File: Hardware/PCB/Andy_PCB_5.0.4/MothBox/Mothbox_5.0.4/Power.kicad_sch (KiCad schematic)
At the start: 50 parts, among them J1 DB141V-2.54-4P, J2 DB141V-2.54-4P, J3 DB141V-2.54-4P, Q1 AP30P30Q, Q10 AP30P30Q, Q2 AO3400A, Q8 AP30P30Q, SW2 KH-6X6X5H-STM, U1 Place Holder voltage regulator, U2 XL4015E1, U3 INA219BIDCNT

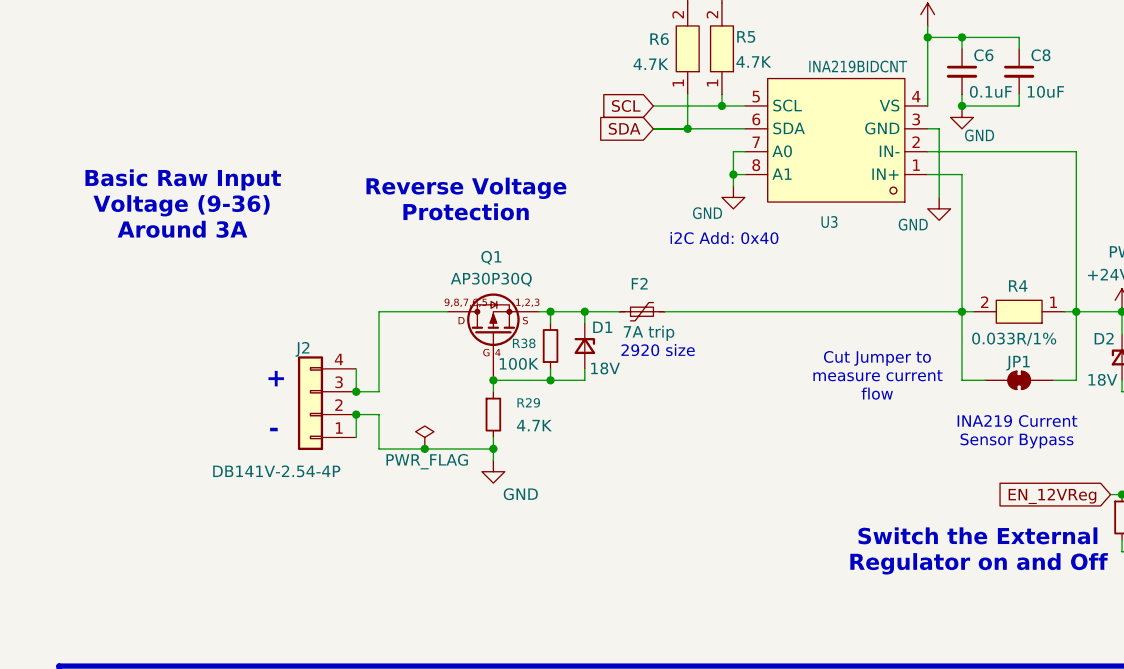
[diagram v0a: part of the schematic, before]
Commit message: v5.0.4 schematic and PCB done. Ready for review
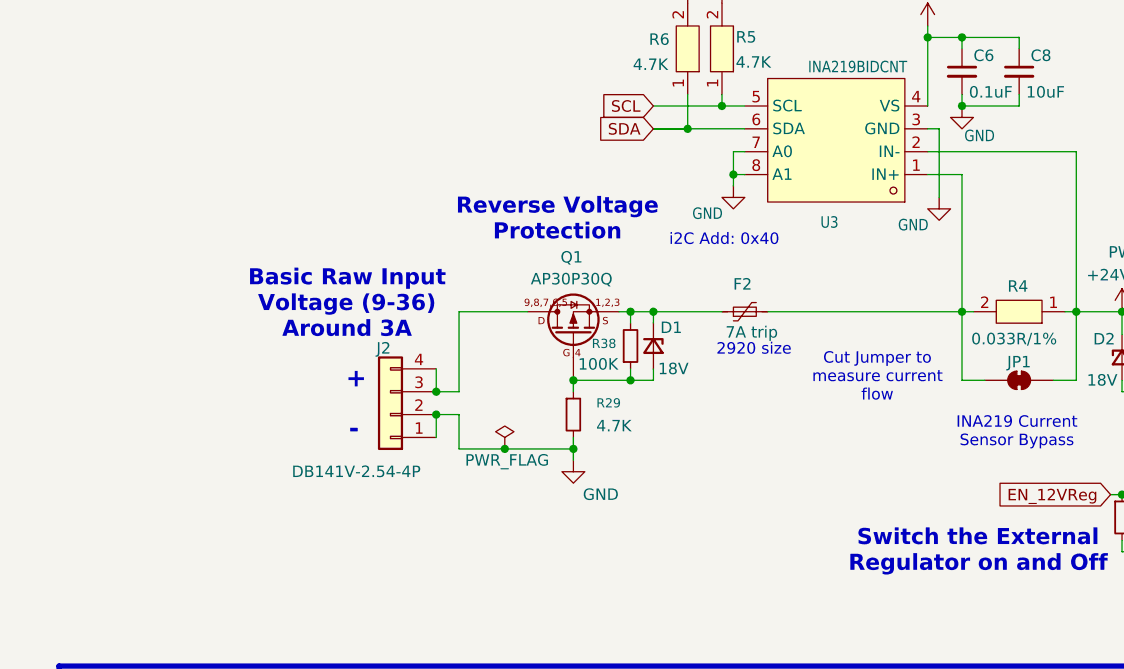
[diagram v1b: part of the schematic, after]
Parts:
- D1, D2, D4: LCSC_Part C22395529 -> C382948
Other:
- moved on the sheet: D1, F2, J2, Q1, R29, R38
